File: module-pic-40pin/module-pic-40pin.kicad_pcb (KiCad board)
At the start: 2 copper layers, 93 x 61.9 mm, 27 parts, among them J1 input_power, J2 ANALOG, J3 icsp, J4 PORTB, J5 PORTC, J6 Conn_02x04_Odd_Even, J7 RB0_CONN, J8 PORTD, SW1 reset, SW2 EXT_INT0, U1 PIC16F877A-IP, Y1 20MHz

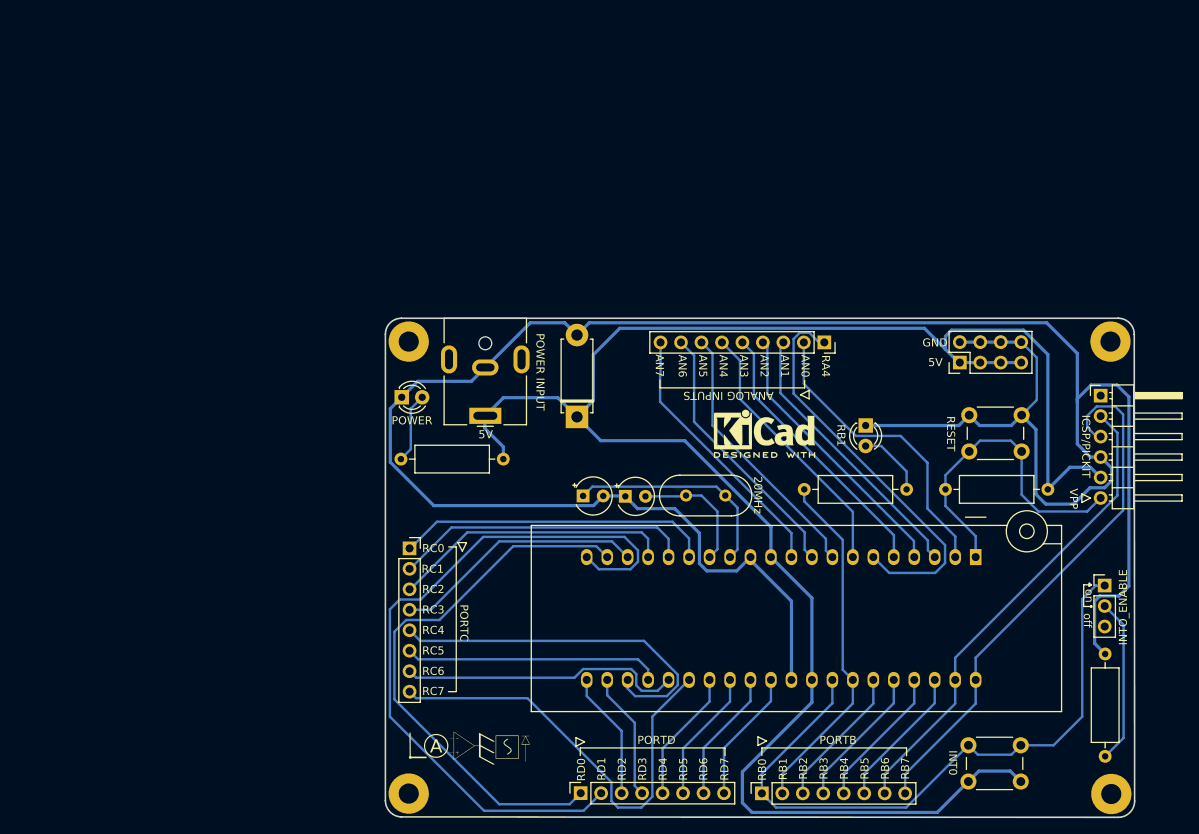
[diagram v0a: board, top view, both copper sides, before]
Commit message: update module-pic-40pin
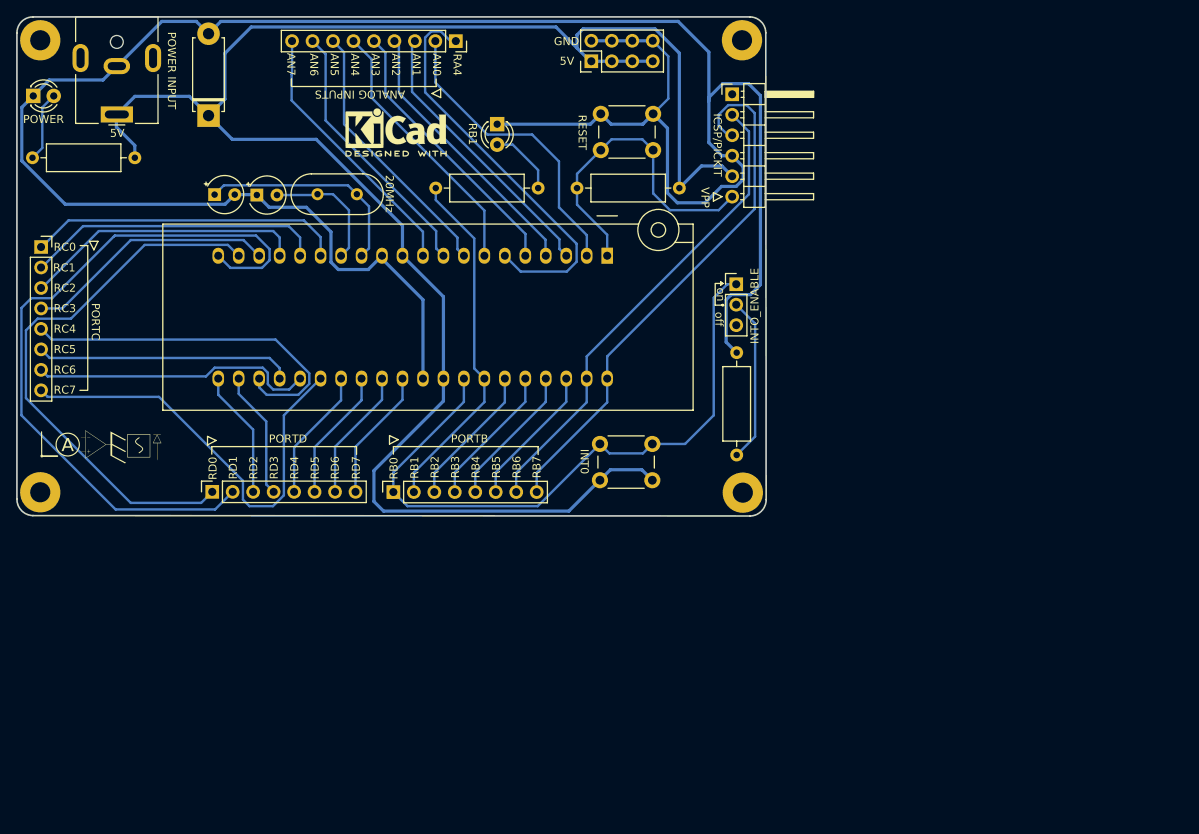
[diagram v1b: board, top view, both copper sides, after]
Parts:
- moved R4 59.1 mm to (123.9, 50.6)
- moved Y1 59.1 mm to (96.5, 51.4)
- moved C2 59.1 mm to (89.0, 51.5)
- moved R3 59.1 mm to (61.1, 46.8)
- moved REF** 59.1 mm to (62.1, 32.3)
- moved REF** 59.1 mm to (62.1, 88.3)
- moved C1 59.1 mm to (83.7, 51.4)
- moved D1 59.1 mm to (118.8, 42.7)
- moved D2 59.1 mm to (61.2, 39.2)
- moved D3 59.1 mm to (83.0, 41.6)
- moved G*** 59.1 mm to (69.6, 82.7)
- moved J1 59.1 mm to (71.6, 41.5)
- moved J2 59.1 mm to (113.6, 32.4)
- moved J3 59.1 mm to (147.9, 39.0)
- moved J6 59.1 mm to (130.5, 34.9)
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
